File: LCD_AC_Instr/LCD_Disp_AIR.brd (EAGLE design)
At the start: 58.4 x 59.1 mm, 30 parts, among them J1 12V input, Q1 16MHz, SW1 ENCODER_SW1-PEC12, U1 ATMEGA328P, U2 5V, U3 +5V

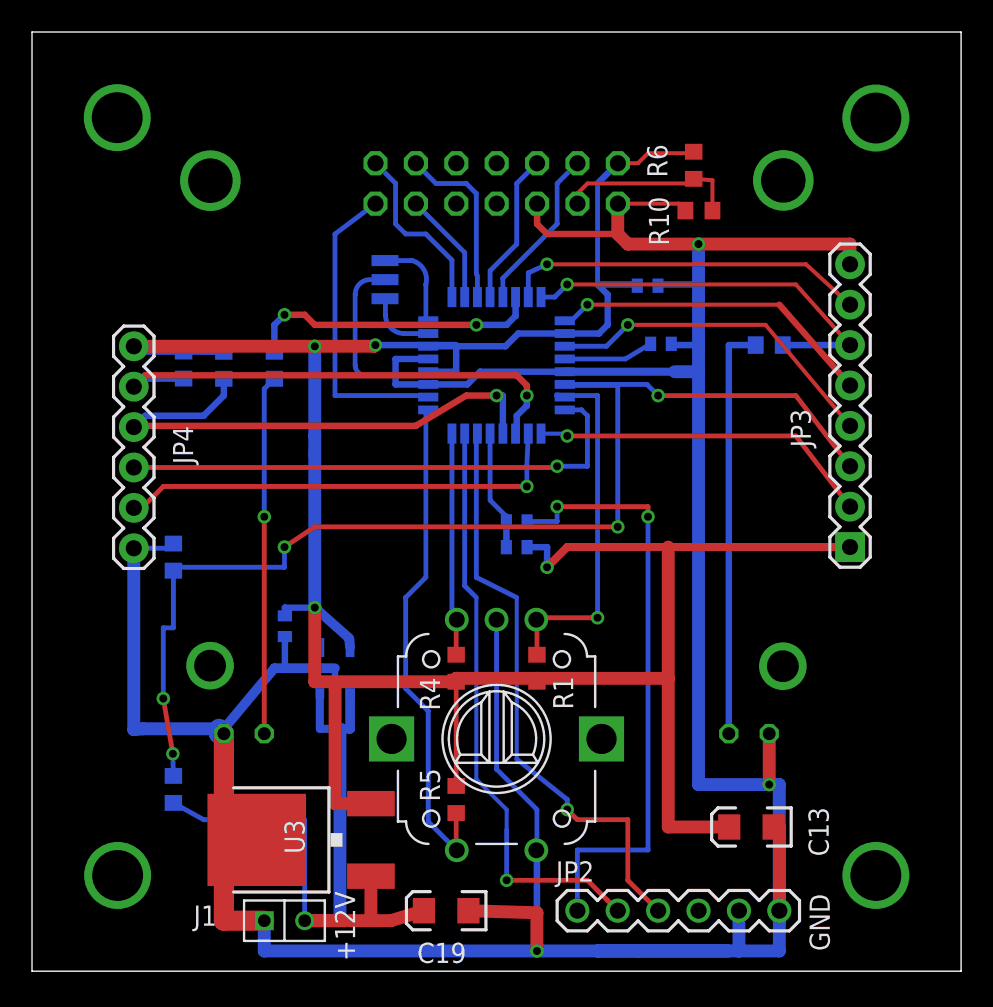
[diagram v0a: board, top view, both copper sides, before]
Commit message: Revised to rev 0.1
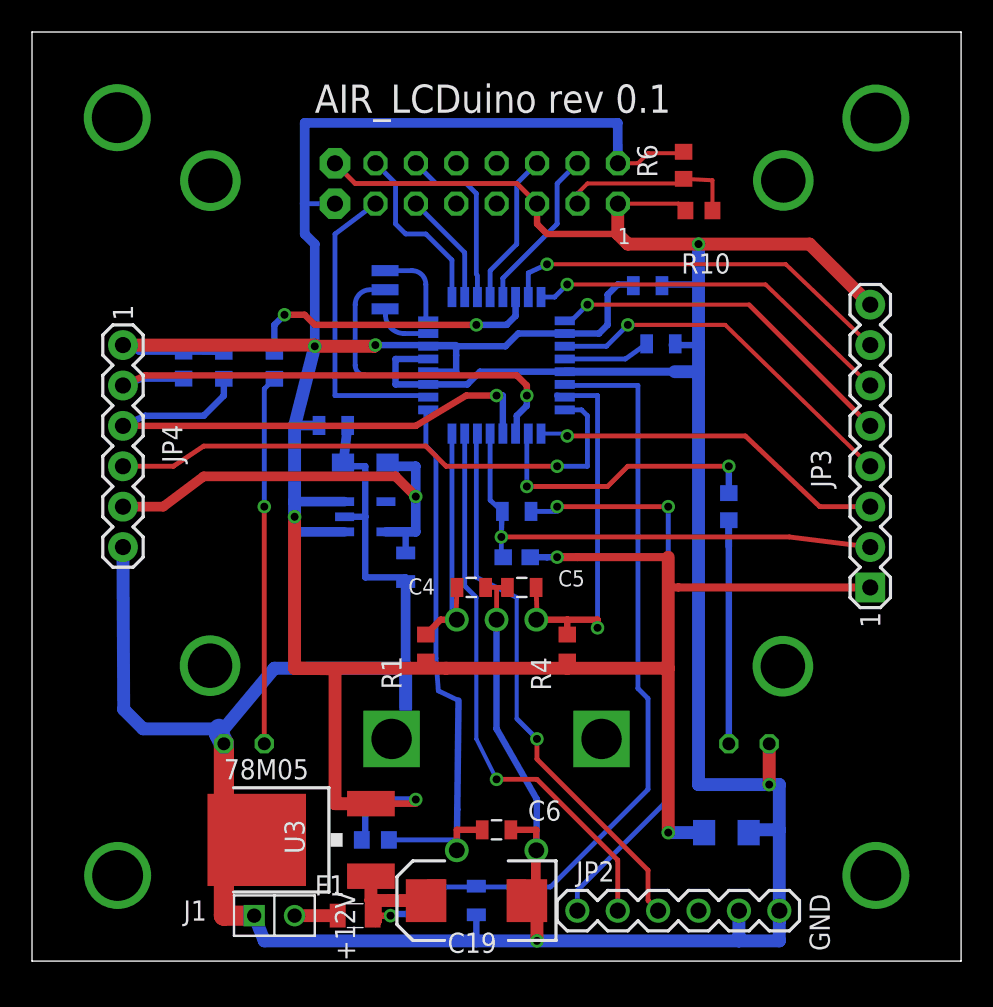
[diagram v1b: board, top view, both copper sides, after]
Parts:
- removed U2: 5V, SparkFun:SOT23-5
- added C4, C5, C6, C8, C9: 0.1uF, SparkFun:0805
- added C7: 10uF, SparkFun:EIA3216
- added F1: (no value), dp_devices:PTC0805
- added IC3: TC10553.3V, 1AA_Stofer:SOT23-5
- added LCD-BL: (no value), 1AA_Stofer:1X02
- C1, C10, C2, C3: device SparkFun:C0402 -> SparkFun:0805
- C19: device SparkFun:EIA3216 -> SparkFun:EIA7343
- R10: value 10K -> 120
- R11: value 10K -> 14K
- R12: value 5K -> 6.8K
- R2, R3: value 330 -> 470
- R6: value 10K -> (none)
- R9: device SparkFun:C0402 -> SparkFun:0603
- U1: value ATMEGA328P -> ATMEGA328P-AU(R)
- U3: value +5V -> 78M05
- moved R12 30.5 mm to (33.0, 6.35), turned to 90 degrees
- moved R11 17.9 mm to (27.9, 6.35)
- moved C10 13.0 mm to (21.5, 36.2), turned to 180 degrees
- moved R3 10.5 mm to (46.4, 31.1), turned to 90 degrees
- moved R1 7.10 mm to (27.3, 22.2)
- moved R4 7.10 mm to (36.2, 22.2)
- moved R5 5.68 mm to (24.1, 10.2), flipped to the bottom, turned to 0 degrees
- moved JP3 2.84 mm to (55.2, 26.0)
- moved C19 2.01 mm to (30.5, 6.34)
- moved C13 1.61 mm to (46.2, 10.6), flipped to the bottom, turned to 0 degrees
- moved J1 0.71 mm to (17.8, 5.40)
- moved JP4 0.69 mm to (8.26, 41.3)
- moved R6 0.64 mm to (43.5, 52.6)
- moved R9 0.64 mm to (33.0, 27.9)
- moved C2 0.63 mm to (33.0, 30.8)
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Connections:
- removed net D2_PD2: R4.2, SW1.B, U1.32
- removed net D3_PD3: R5.1, SW1.P2, U1.1
- new net D2_PD2(INT0): C4.2, R1.1, SW1.A, U1.32
- new net D3_PD3(INT1): C6.2, R5.1, SW1.P1, U1.1
- new net N$11: F1.1, J1.2
- new net V3_3V: C7.A, C8.1, IC3.5, JP4.5
- net 12V_INPUT: now also F1.2; no longer J1.2, U2.1, U2.3
- net 5V: now also IC3.1, IC3.3, LCD-BL.2; no longer U2.5
- net A0_PC0: now also C5.2, R4.2, SW1.B; no longer R1.1, SW1.A
- net A2_PC2: now also JP3.3; no longer JP3.2
- net A3_PC3: now also R3.2; no longer JP4.5
- net ADC7: now also C9.1; no longer JP3.3
- net D12_PB4_MISO: no longer R3.2
- net GND: now also C4.1, C5.1, C6.1, C7.C, C8.2, C9.2, IC3.2, LCD-BL.1, SW1.P2; no longer SW1.P1, U2.2
- net RESET: now also JP3.2
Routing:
- net 5V: track 171.4 -> 209.9 mm, vias 4 -> 6
- net D3_PD3(INT1): track 0.00 -> 38.0 mm
- net 12V_INPUT: track 46.5 -> 10.6 mm, vias 0 -> 1
- net D3_PD3: track 32.1 -> 0.00 mm
- net ADC7: track 76.1 -> 46.3 mm, vias 5 -> 0
- net V3_3V: track 0.00 -> 28.7 mm, vias 0 -> 1
- net RESET: track 7.58 -> 33.1 mm, vias 0 -> 1
- net GND: track 247.9 -> 273.0 mm
- net D2_PD2(INT0): track 0.00 -> 16.4 mm
- net D2_PD2: track 14.2 -> 0.00 mm
- net N$15: track 26.1 -> 15.7 mm
- net A3_PC3: track 28.6 -> 18.3 mm, vias 1 -> 2
- net N$11: track 0.00 -> 2.71 mm
- net D11_PB3_MOSI: track 22.9 -> 25.2 mm
- net D13_PB5_SCK: track 20.7 -> 22.8 mm
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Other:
- board size 58.4 x 59.1 mm -> 58.4 x 58.4 mm
- board text added: "1"
- board text added: "AIR_LCDuino rev 0.1"
- board text added: "RV-Builders Products"
